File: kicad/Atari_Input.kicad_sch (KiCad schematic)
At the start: 12 parts

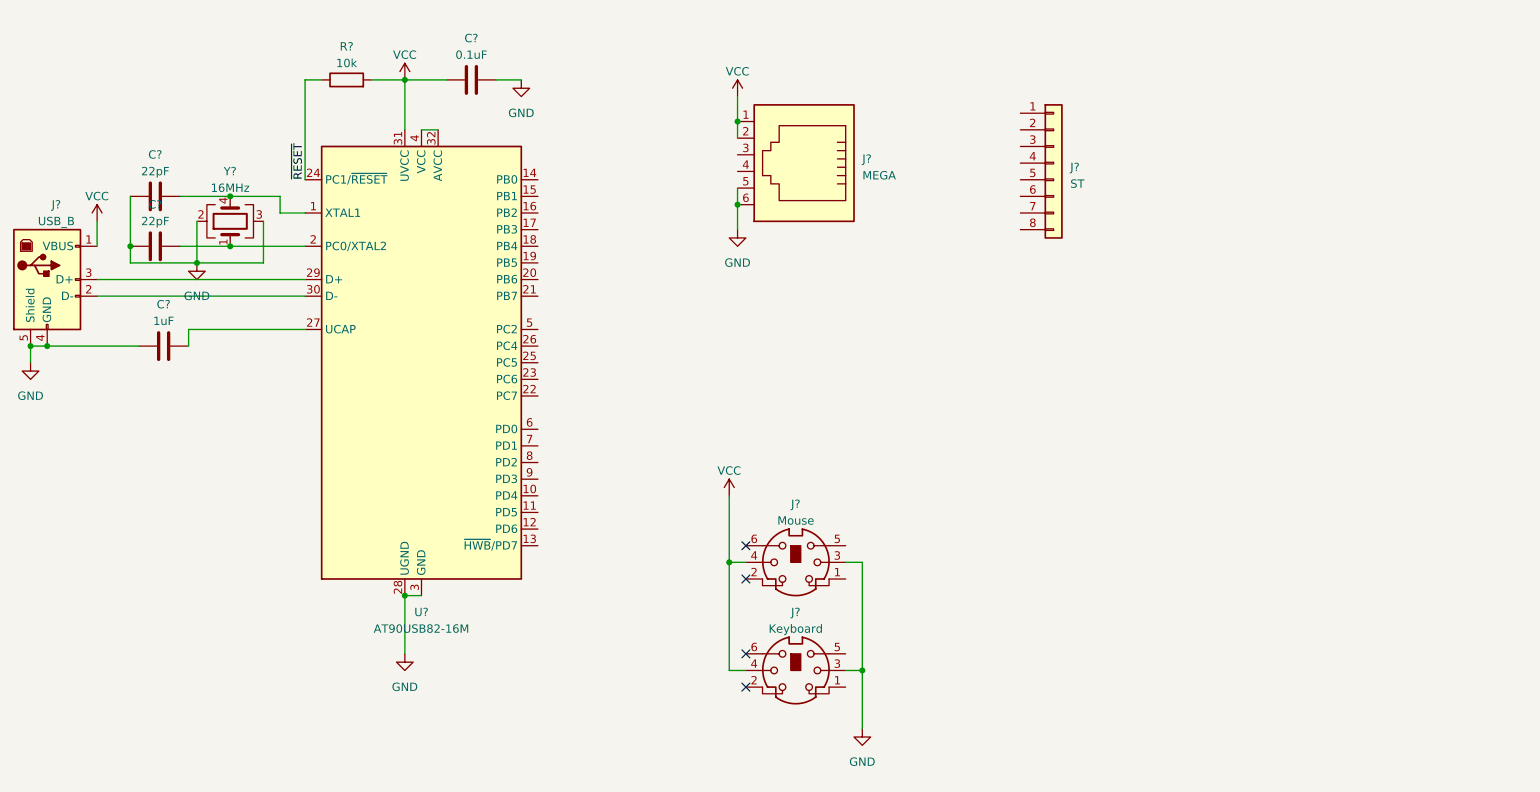
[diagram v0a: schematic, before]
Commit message: a
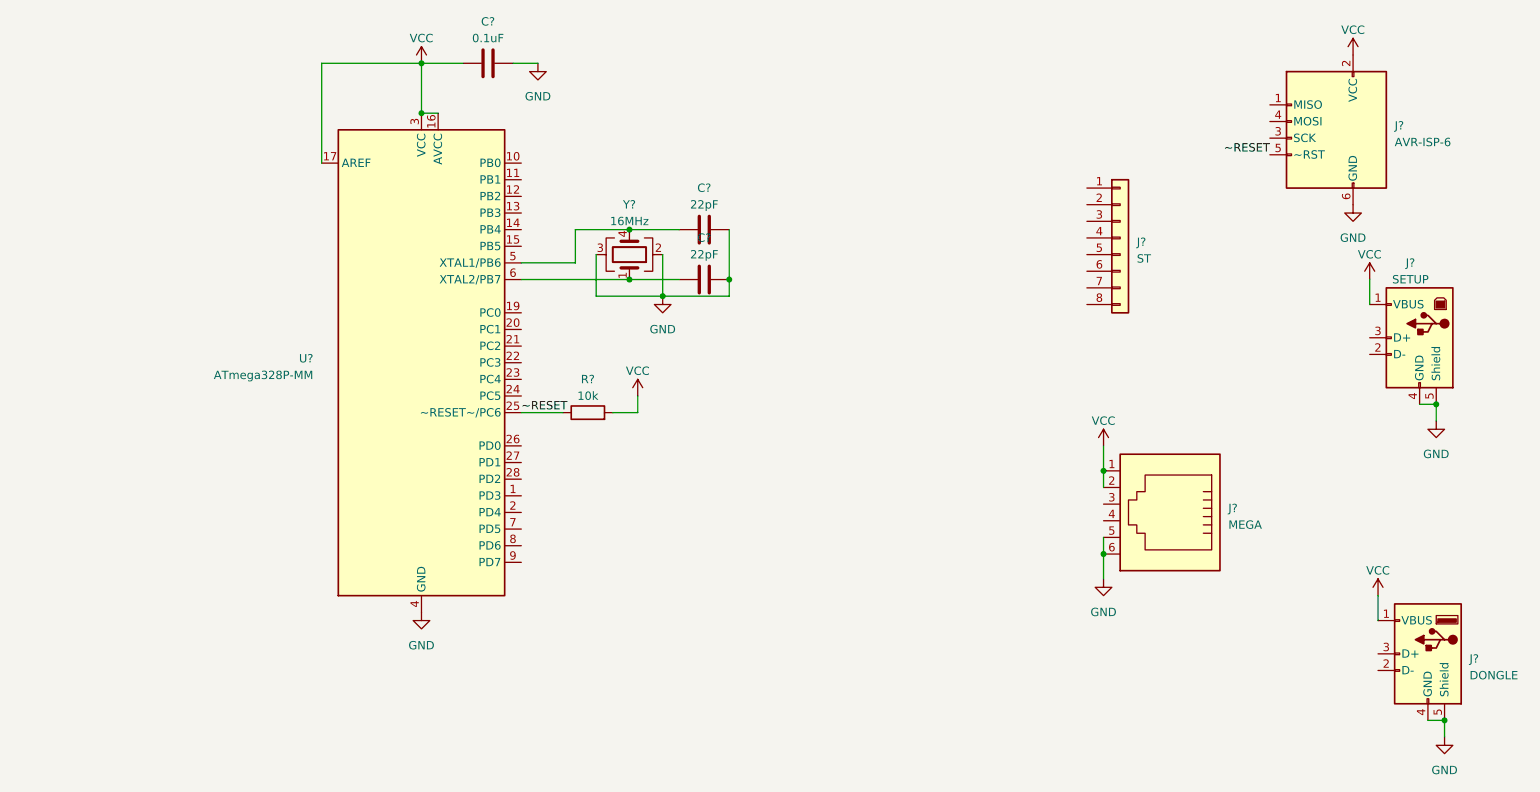
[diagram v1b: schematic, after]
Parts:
- removed C?: 1uF, symbol Device:C
- removed J?: Keyboard, symbol Connector:Mini-DIN-6
- removed J?: Mouse, symbol Connector:Mini-DIN-6
- removed J?: USB_B, symbol Connector:USB_B
- removed R?: 10k, symbol Device:R
- removed U?: AT90USB82-16M, Package_DFN_QFN:QFN-32-1EP_5x5mm_P0.5mm_EP3.6x3.6mm, symbol MCU_Microchip_AVR:AT90USB82-16M
- added J?: SETUP, symbol Connector:USB_B
- added J?: AVR-ISP-6, Connector_IDC:IDC-Header_2x03_P2.54mm_Vertical, symbol Connector:AVR-ISP-6
- added J?: DONGLE, Connector_USB:USB_A_Molex_67643_Horizontal, symbol Connector:USB_A
- added R?: 10k, symbol Device:R
- added U?: ATmega328P-MM, Package_DFN_QFN:QFN-28-1EP_4x4mm_P0.45mm_EP2.4x2.4mm, symbol MCU_Microchip_ATmega:ATmega328P-MM
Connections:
- net GND: now also J?.4 (GND), J?.4 (GND), J?.5 (Shield), J?.5 (Shield), J?.6 (GND), U?.18 (GND), U?.29 (GND), U?.4 (GND)
- net VCC: now also J?.1 (VBUS), J?.1 (VBUS), J?.2 (VCC), R?.2, U?.16 (AVCC), U?.17 (AREF), U?.3 (VCC)
- net ~RESET: now also J?.5 (~RST), R?.1, U?.25 (~RESET~/PC6)
- net at C?.2, Y?.4: now also U?.5 (XTAL1/PB6)
- net at C?.2, Y?.1: now also U?.6 (XTAL2/PB7)
- no-connect marks 4 -> 0
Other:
- moved on the sheet: C?, J?, Y?
